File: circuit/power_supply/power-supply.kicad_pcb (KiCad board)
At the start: 2 copper layers, 66 x 38.7 mm, 21 parts, among them P1 CONN_2, U1 MCS34063A

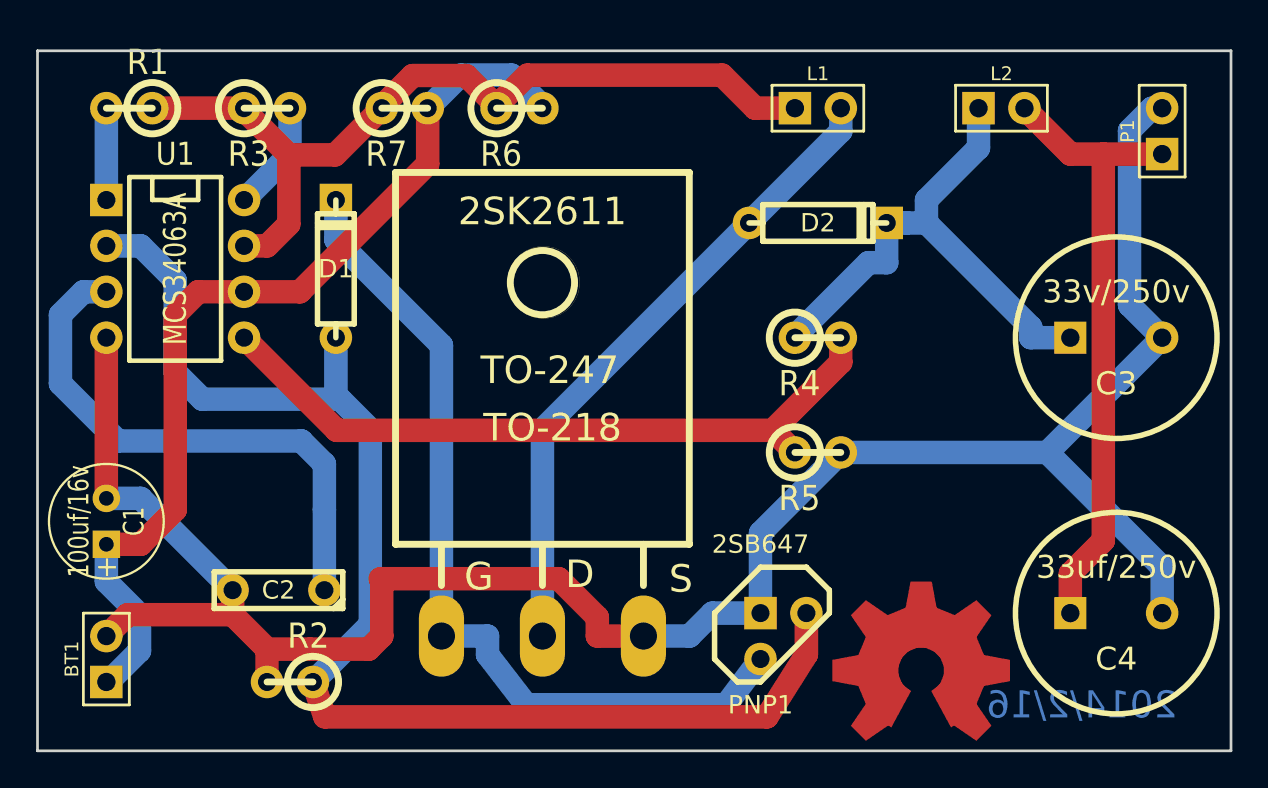
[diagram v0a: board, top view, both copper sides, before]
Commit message: Remove the coper zone
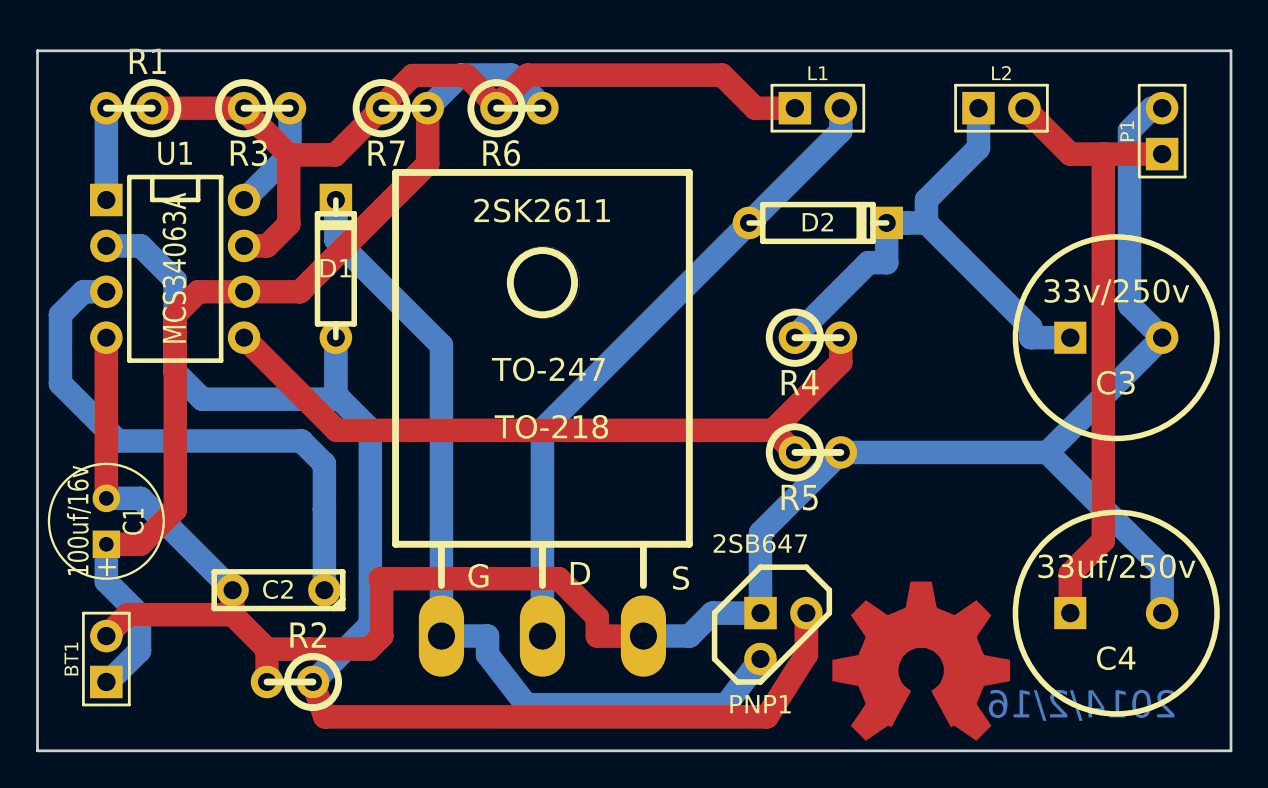
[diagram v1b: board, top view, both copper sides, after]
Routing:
- removed copper zone on B.Cu, net (none)
- removed copper zone on F.Cu, net (none)
